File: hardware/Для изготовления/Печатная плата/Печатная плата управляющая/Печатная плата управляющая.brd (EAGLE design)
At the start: 100 x 114.3 mm, 23 parts, among them J1 POWER_JACK, Q1 IRF540

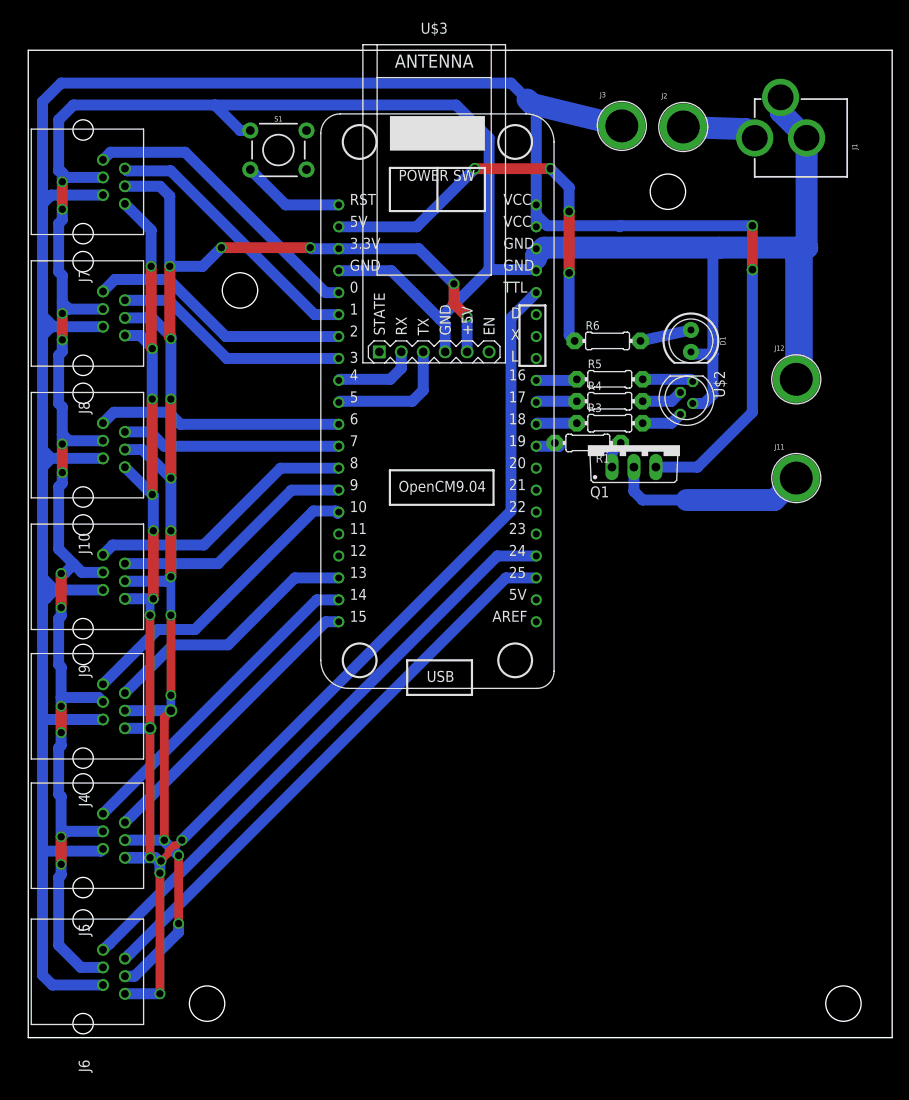
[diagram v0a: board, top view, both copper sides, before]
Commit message: изменена управляющая плата
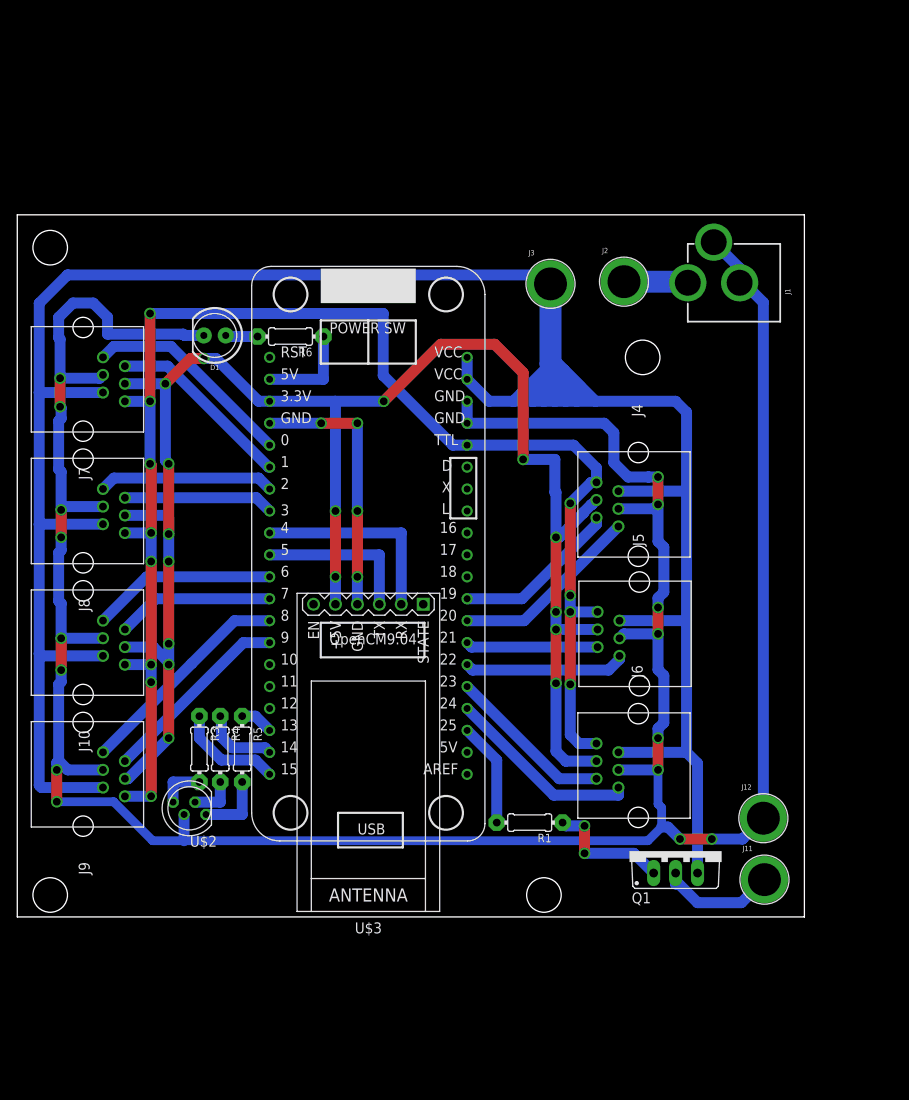
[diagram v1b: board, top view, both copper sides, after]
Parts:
- removed S1: reset_button, SparkFun-Switches:TACTILE_SWITCH_PTH_6.0MM
- R1: value 330 -> 100
- moved U$2 74.6 mm to (18.7, -0.13), turned to 180 degrees
- moved J6 68.6 mm to (70.6, 4.83), turned to 90 degrees
- moved J5 68.5 mm to (70.7, 20.1), turned to 90 degrees
- moved J4 68.4 mm to (70.6, 35.1), turned to 90 degrees
- moved U$3 64.0 mm to (39.4, 6.35), turned to 180 degrees
- moved R3 60.7 mm to (19.8, 6.73), turned to 270 degrees
- moved R4 60.4 mm to (22.2, 6.73), turned to 270 degrees
- moved R5 60.3 mm to (24.8, 6.73), turned to 270 degrees
- moved D1 55.1 mm to (21.6, 54.6), turned to 180 degrees
- moved J12 50.9 mm to (85.1, -1.27)
- moved Q1 47.2 mm to (74.9, -5.08)
- moved J11 46.6 mm to (85.2, -8.38)
- moved R1 44.5 mm to (58.0, -1.78)
- moved R6 36.7 mm to (30.4, 54.5), turned to 180 degrees
- moved J9 22.9 mm to (6.35, 3.81)
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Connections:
- removed net RST: S1.3, U$1.RST
- net BLUE: now also U$1.13; no longer U$1.16
- net ENCODER_X_1: now also U$1.20; no longer U$1.10
- net ENCODER_X_2: now also U$1.22; no longer U$1.14
- net ENDSTOP_X_1: now also U$1.19; no longer U$1.13
- net ENDSTOP_X_2: now also U$1.21; no longer U$1.15
- net ENDSTOP_Y: now also U$1.23; no longer U$1.25
- net GND: no longer S1.1
- net GREEN: now also U$1.14; no longer U$1.17
- net PUMP: now also U$1.25; no longer U$1.19
- net RED: now also U$1.15; no longer U$1.18
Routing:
- net ENDSTOP_Y: track 65.9 -> 19.4 mm
- net ENCODER_Y: track 69.0 -> 22.6 mm
- net 5V: track 48.4 -> 11.2 mm, vias 4 -> 0
- net RX/TX: track 201.7 -> 170.4 mm, vias 13 -> 12
- net 3.3V: track 172.8 -> 202.1 mm
- net GND: track 348.5 -> 372.3 mm, vias 12 -> 20
- net ENDSTOP_X_2: track 34.4 -> 15.3 mm
- net ENCODER_X_2: track 37.5 -> 18.8 mm
- net TX2: track 9.72 -> 23.5 mm
- net ENCODER_X_1: track 35.8 -> 22.0 mm
- net RST: track 11.9 -> 0.00 mm
- net N$3: track 3.21 -> 14.8 mm, vias 0 -> 2
- net ENDSTOP_X_1: track 30.3 -> 19.3 mm
- net ENCODER_Z_2: track 30.6 -> 20.3 mm
- net ENDSTOP_Z_2: track 27.5 -> 17.4 mm
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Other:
- board size 100 x 114.3 mm -> 91.1 x 81.3 mm
